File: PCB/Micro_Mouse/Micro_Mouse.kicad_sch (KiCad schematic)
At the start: 12 parts, among them J1 Motor Battery Pack, J3 MOT_1/ENC_1, J4 MOT2/ENC_2, J5 TOF, J6 IR_1, J7 IR_2, J8 IMU, Q1 PMOS, U1 TB6612FNG

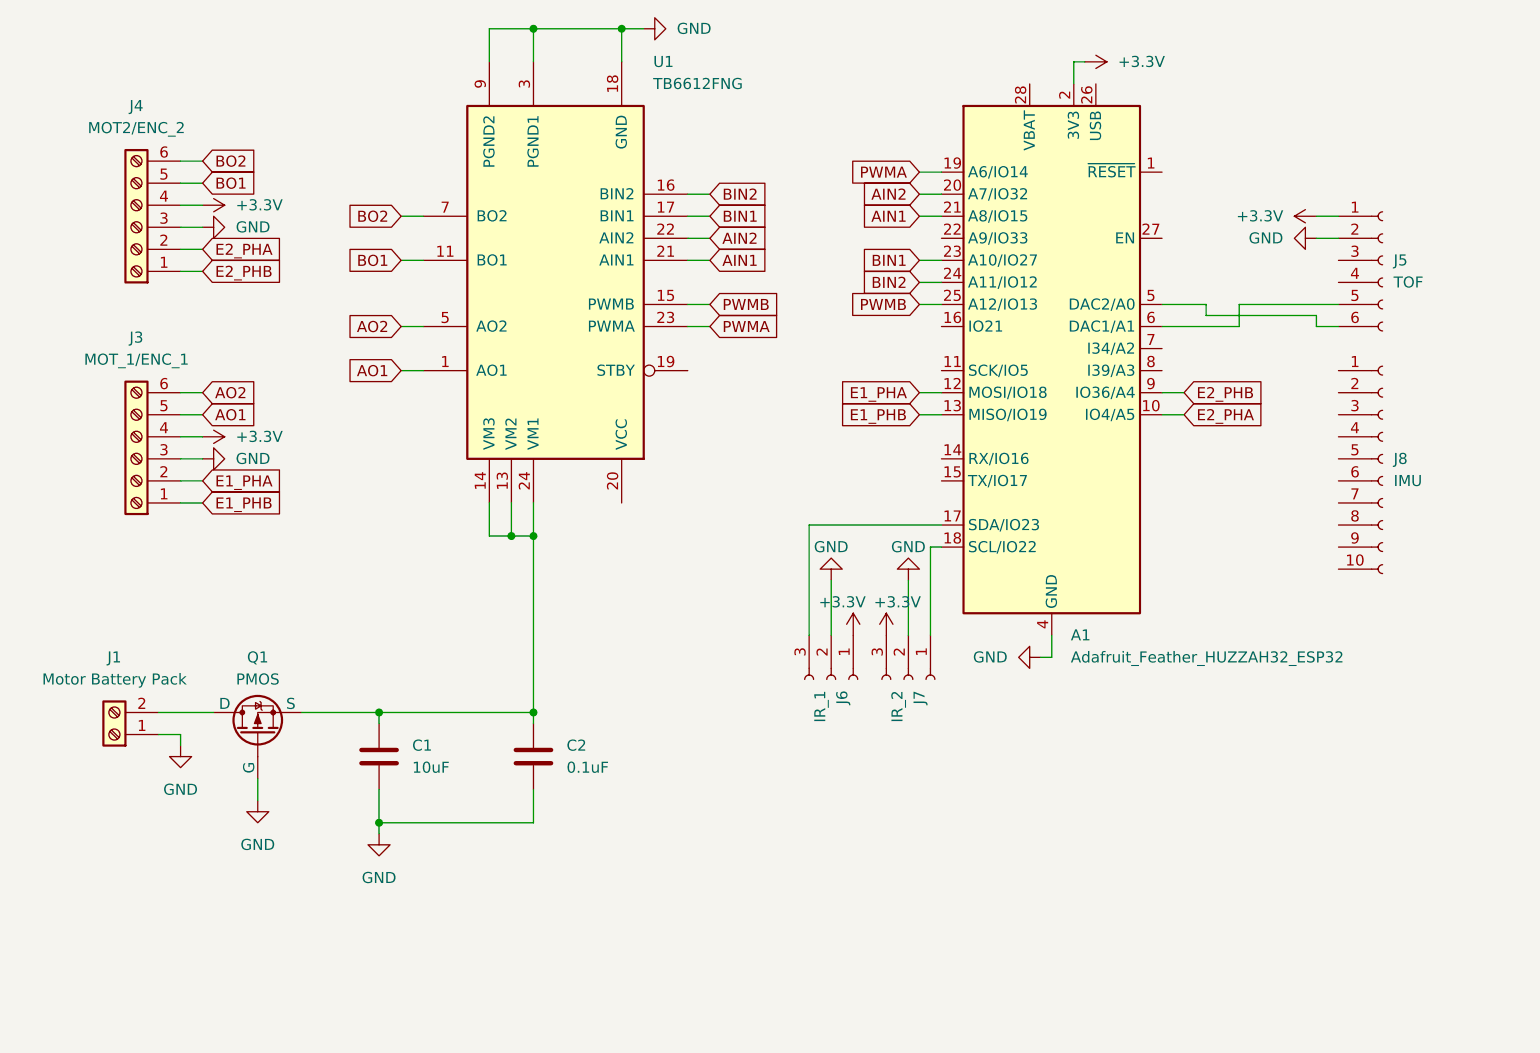
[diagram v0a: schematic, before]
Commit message: Add files via upload
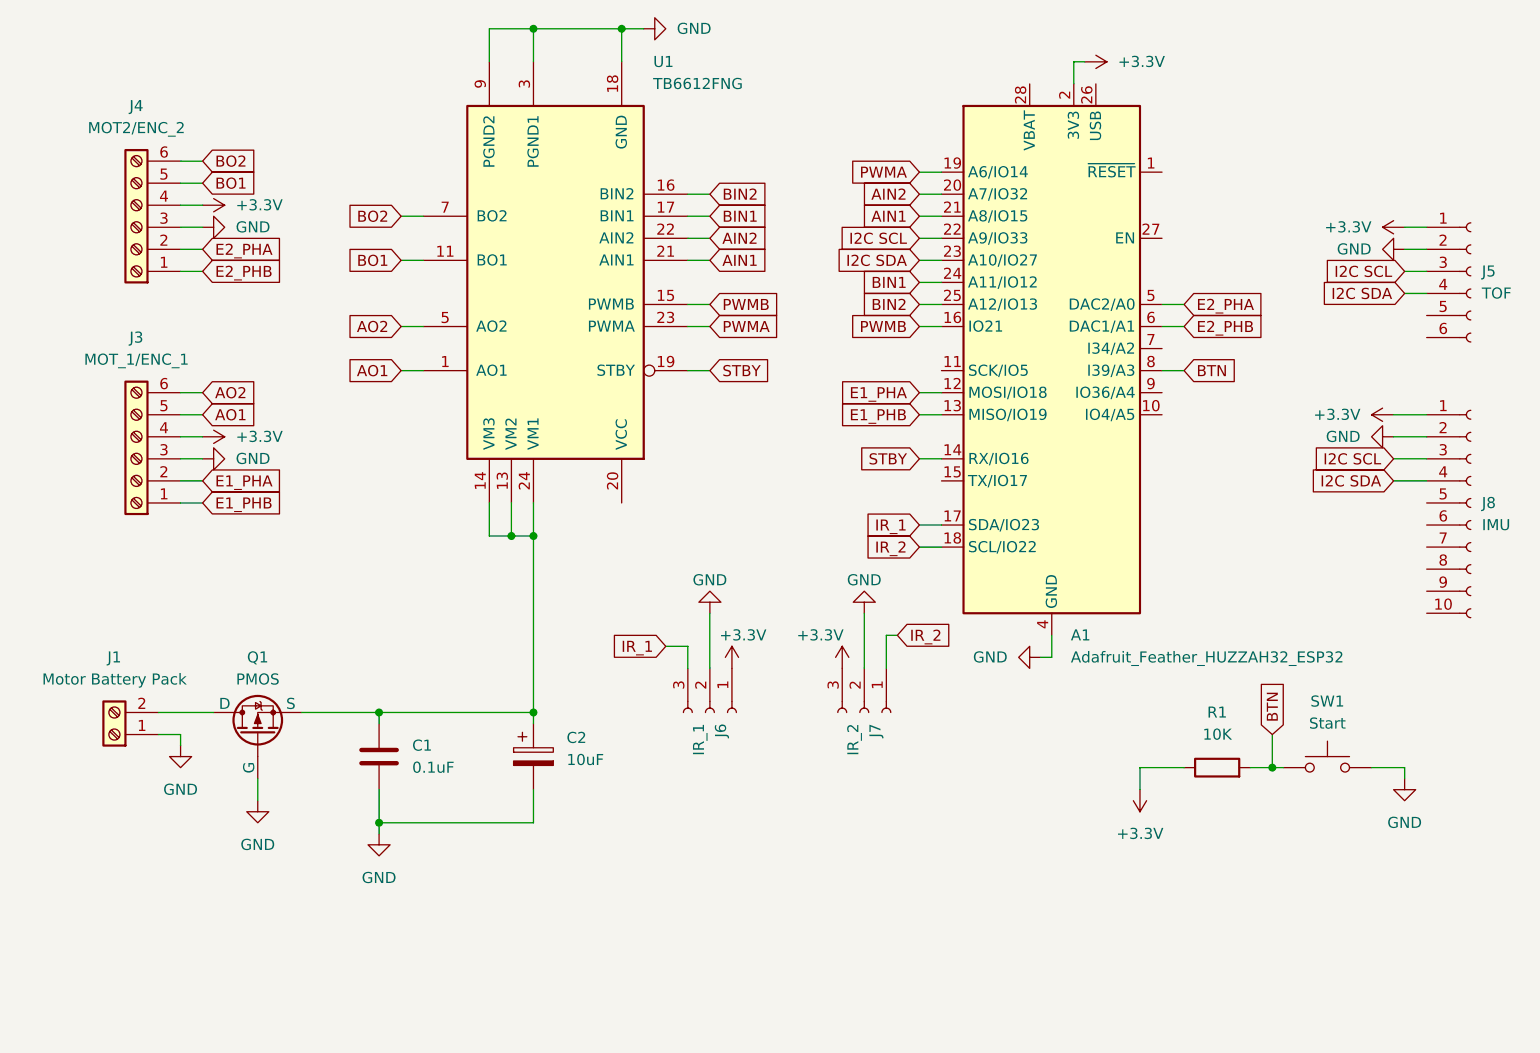
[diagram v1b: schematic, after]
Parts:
- removed C2: 0.1uF, symbol Device:C
- added C2: 10uF, Capacitor_SMD:CP_Elec_3x5.3, symbol Device:C_Polarized
- added R1: 10K, Resistor_SMD:R_0805_2012Metric, symbol Device:R
- added SW1: Start, Button_Switch_SMD:SW_Push_1P1T_NO_CK_KSC6xxJ, symbol Switch:SW_Push
- C1: value 10uF -> 0.1uF; footprint (none) -> Capacitor_SMD:CP_Elec_3x5.3
- J1: footprint TerminalBlock_Phoenix:TerminalBlock_Phoenix_MPT-0,5-2-2.54_1x02_P2.54mm_Horizontal -> Connector_JST:JST_EH_B2B-EH-A_1x02_P2.50mm_Vertical
- Q1: footprint (none) -> Package_TO_SOT_SMD:TO-252-2
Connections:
- net +3.3V: now also J8.1 (Pin_1), R1.1
- net BIN1: now also A1.24 (A11/IO12); no longer A1.23 (A10/IO27)
- net BIN2: now also A1.25 (A12/IO13); no longer A1.24 (A11/IO12)
- net E2_PHA: now also A1.5 (DAC2/A0); no longer A1.10 (IO4/A5)
- net E2_PHB: now also A1.6 (DAC1/A1); no longer A1.9 (IO36/A4)
- net GND: now also J8.2 (Pin_2), C2.2, SW1.2
- net PWMB: now also A1.16 (IO21); no longer A1.25 (A12/IO13)
- net STBY: now reaches A1.14 (RX/IO16)
- net STBY: now also U1.19 (STBY)
- net IR_1: now reaches A1.17 (SDA/IO23), J6.3 (Pin_3)
- net IR_2: now reaches A1.18 (SCL/IO22), J7.1 (Pin_1)
- net I2C SCL: now reaches A1.22 (A9/IO33)
- net I2C SCL: now also J5.3 (Pin_3), J8.3 (Pin_3)
- net at J5.6 (Pin_6): no longer A1.5 (DAC2/A0)
- net at J5.5 (Pin_5): no longer A1.6 (DAC1/A1)
- net BTN: now reaches A1.8 (I39/A3)
- net BTN: now also R1.2, SW1.1
- net at C1.1, Q1.3 (S), U1.13 (VM2)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: now also C2.1
- net I2C SDA: now reaches J8.4 (Pin_4)
- net I2C SDA: now also A1.23 (A10/IO27), J5.4 (Pin_4)
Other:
- title: (none) -> Micro Mouse: Santana, West
- moved on the sheet: J5, J6, J7, J8

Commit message: Add files via upload
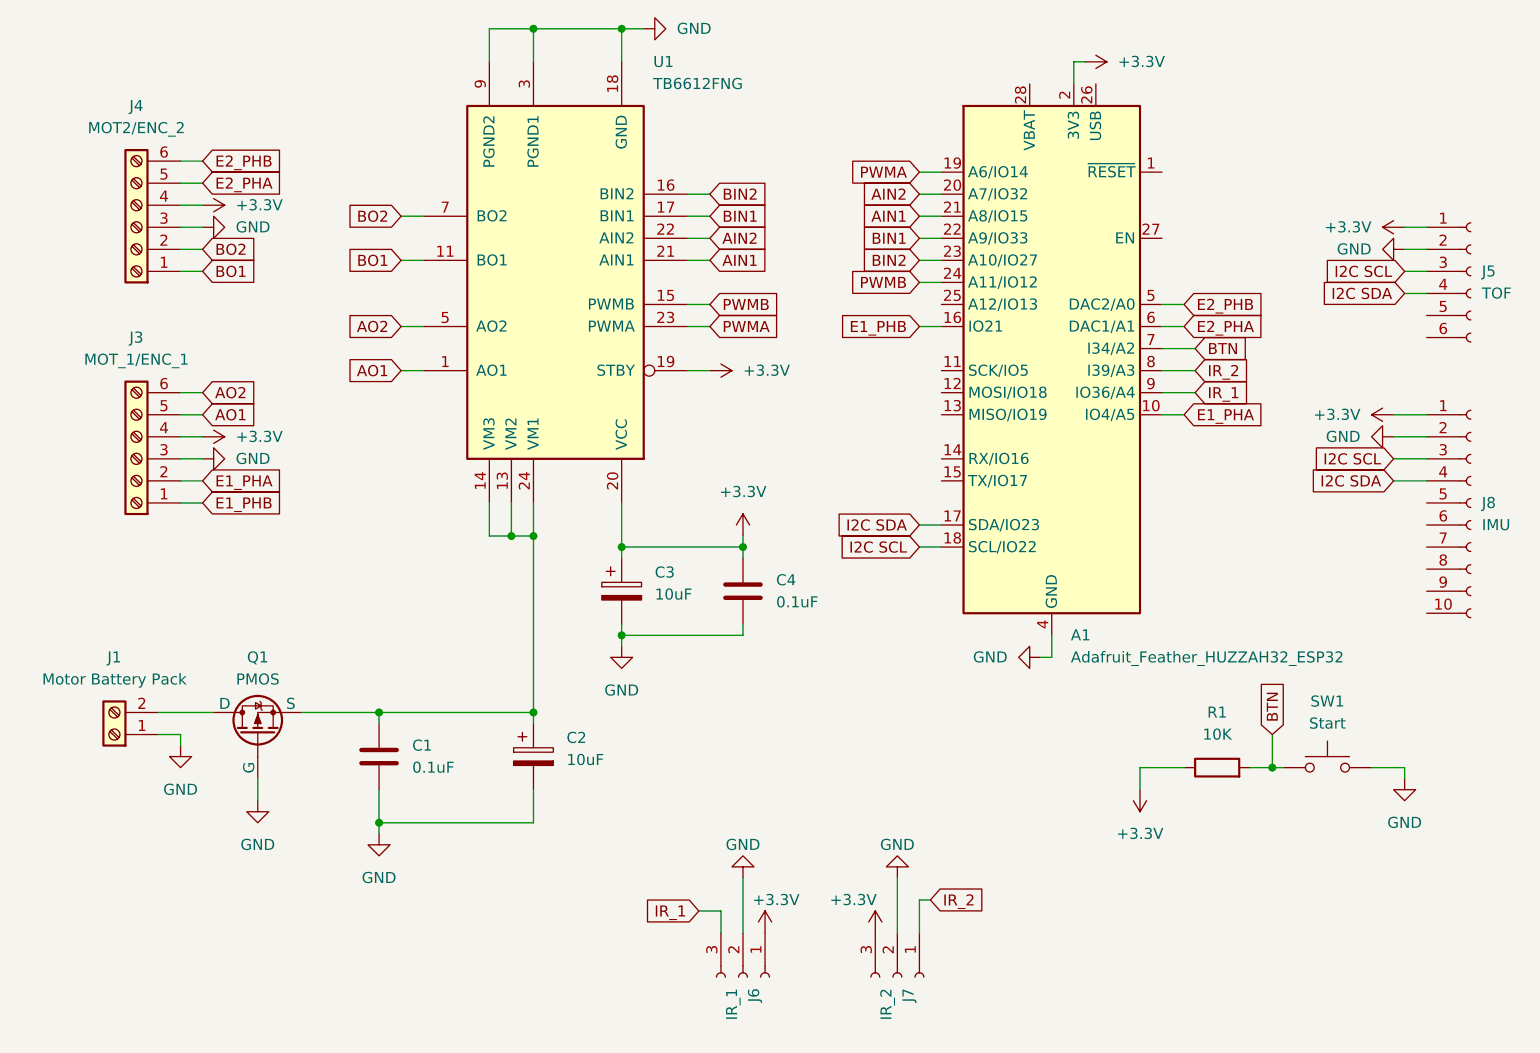
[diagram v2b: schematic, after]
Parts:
- added C3: 10uF, Capacitor_SMD:CP_Elec_3x5.3, symbol Device:C_Polarized
- added C4: 0.1uF, Capacitor_SMD:C_0805_2012Metric_Pad1.18x1.45mm_HandSolder, symbol Device:C
- C1: footprint Capacitor_SMD:CP_Elec_3x5.3 -> Capacitor_SMD:C_0805_2012Metric_Pad1.18x1.45mm_HandSolder
- Q1: footprint Package_TO_SOT_SMD:TO-252-2 -> Package_TO_SOT_SMD:TO-252-3_TabPin2
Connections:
- net +3.3V: now also U1.19 (STBY), U1.20 (VCC), C3.1, C4.1
- net BIN1: now also A1.22 (A9/IO33); no longer A1.24 (A11/IO12)
- net BIN2: now also A1.23 (A10/IO27); no longer A1.25 (A12/IO13)
- net BO1: now also J4.1 (Pin_1); no longer J4.5 (Pin_5)
- net BO2: now also J4.2 (Pin_2); no longer J4.6 (Pin_6)
- net BTN: now also A1.7 (I34/A2); no longer A1.8 (I39/A3)
- net E1_PHA: now also A1.10 (IO4/A5); no longer A1.12 (MOSI/IO18)
- net E1_PHB: now also A1.16 (IO21); no longer A1.13 (MISO/IO19)
- net E2_PHA: now also A1.6 (DAC1/A1), J4.5 (Pin_5); no longer A1.5 (DAC2/A0), J4.2 (Pin_2)
- net E2_PHB: now also A1.5 (DAC2/A0), J4.6 (Pin_6); no longer A1.6 (DAC1/A1), J4.1 (Pin_1)
- net GND: now also C3.2, C4.2
- net I2C SCL: now also A1.18 (SCL/IO22); no longer A1.22 (A9/IO33)
- net I2C SDA: now also A1.17 (SDA/IO23); no longer A1.23 (A10/IO27)
- net IR_1: now also A1.9 (IO36/A4); no longer A1.17 (SDA/IO23)
- net IR_2: now also A1.8 (I39/A3); no longer A1.18 (SCL/IO22)
- net PWMB: now also A1.24 (A11/IO12); no longer A1.16 (IO21)
- net STBY: no longer names the net of A1.14 (RX/IO16)
- net STBY: no longer U1.19 (STBY)
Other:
- moved on the sheet: J6, J7

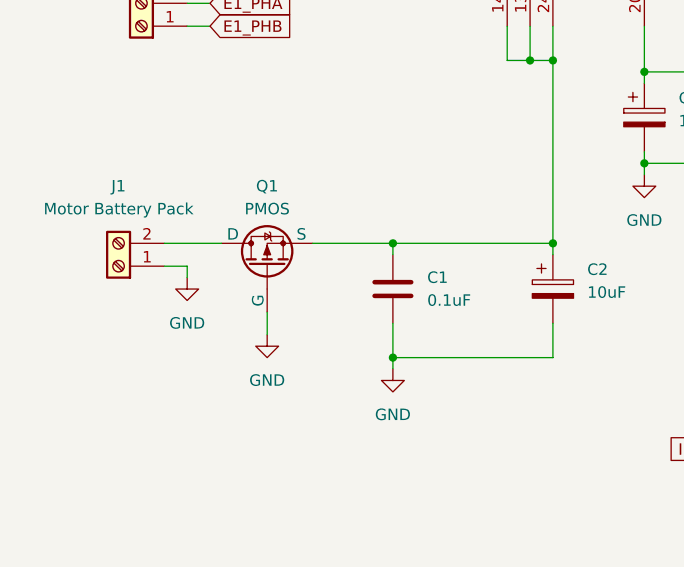
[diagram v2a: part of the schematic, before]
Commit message: Add files via upload
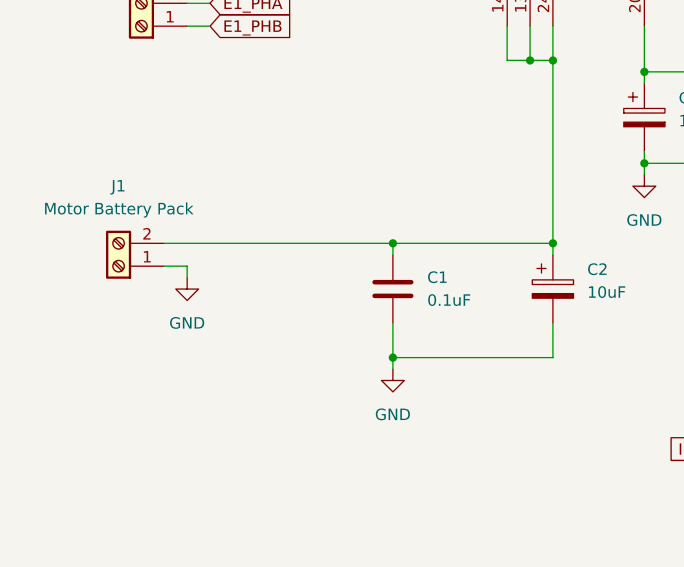
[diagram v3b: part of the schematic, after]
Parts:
- removed Q1: PMOS, Package_TO_SOT_SMD:TO-252-3_TabPin2, symbol Simulation_SPICE:PMOS
- J4: footprint TerminalBlock_Phoenix:TerminalBlock_Phoenix_MPT-0,5-6-2.54_1x06_P2.54mm_Horizontal -> Connector_JST:JST_ZE_B06B-ZESK-1D_1x06_P1.50mm_Vertical
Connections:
- net at C1.1, C2.1, U1.13 (VM2)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: now also J1.2 (Pin_2)
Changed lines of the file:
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@@
     (stroke (width 0) (type default))
   )
-  (wire (pts (xy 59.69 137.16) (xy 68.58 137.16))
+  (wire (pts (xy 43.18 137.16) (xy 68.58 137.16))
     (stroke (width 0) (type default))
   )
@@
     (stroke (width 0) (type default))
   )
-  (wire (pts (xy 43.18 137.16) (xy 49.53 137.16))
-    (stroke (width 0) (type default))
-  )
   (wire (pts (xy 110.49 127) (xy 110.49 128.27))
     (stroke (width 0) (type default))
@@
   )
   (wire (pts (xy 171.45 143.51) (xy 172.72 143.51))
-    (stroke (width 0) (type default))
-  )
-  (wire (pts (xy 54.61 144.78) (xy 54.61 147.32))
     (stroke (width 0) (type default))
   )
@@
     )
   )
-  (symbol (lib_id "power:GND") (at 54.61 147.32 0) (unit 1)
-    (in_bom yes) (on_board yes) (dnp no) (fields_autoplaced)
-    (property "Reference" "#PWR010" (at 54.61 153.67 0)
-      (effects (font (size 1.27 1.27)) hide)
-    )
-    (property "Value" "GND" (at 54.61 152.4 0)
-      (effects (font (size 1.27 1.27)))
-    )
-    (property "Footprint" "" (at 54.61 147.32 0)
-      (effects (font (size 1.27 1.27)) hide)
-    )
-    (property "Datasheet" "" (at 54.61 147.32 0)
-      (effects (font (size 1.27 1.27)) hide)
-    )
-    (pin "1")
-    (instances
-      (project "Micro_Mouse"
-        (path "/2f5422af-6937-496c-8d34-480d197513da"
-          (reference "#PWR010") (unit 1)
-        )
-      )
-    )
-  )
   (symbol (lib_id "Driver_Motor:TB6612FNG") (at 88.9 87.63 180) (unit 1)
     (in_bom yes) (on_board yes) (dnp no) (fields_autoplaced)
@@
     )
   )
-  (symbol (lib_id "Simulation_SPICE:PMOS") (at 54.61 139.7 90) (unit 1)
-    (in_bom yes) (on_board yes) (dnp no) (fields_autoplaced)
-    (property "Reference" "Q1" (at 54.61 130.81 90)
-      (effects (font (size 1.27 1.27)))
-    )
-    (property "Value" "PMOS" (at 54.61 133.35 90)
-      (effects (font (size 1.27 1.27)))
-    )
-    (property "Footprint" "Package_TO_SOT_SMD:TO-252-3_TabPin2" (at 52.07 134.62 0)
-      (effects (font (size 1.27 1.27)) hide)
-    )
-    (property "Datasheet" "https://ngspice.sourceforge.io/docs/ngspice-manual.pdf" (at 67.31 139.7 0)
-      (effects (font (size 1.27 1.27)) hide)
-    )
-    (property "Sim.Device" "PMOS" (at 71.755 139.7 0)
-      (effects (font (size 1.27 1.27)) hide)
-    )
-    (property "Sim.Type" "VDMOS" (at 73.66 139.7 0)
-      (effects (font (size 1.27 1.27)) hide)
-    )
-    (property "Sim.Pins" "1=D 2=G 3=S" (at 69.85 139.7 0)
-      (effects (font (size 1.27 1.27)) hide)
-    )
-    (pin "1")
-    (pin "2")
-    (pin "3")
-    (instances
-      (project "Micro_Mouse"
-        (path "/2f5422af-6937-496c-8d34-480d197513da"
-          (reference "Q1") (unit 1)
-        )
-      )
-    )
-  )
   (symbol (lib_id "Switch:SW_Push") (at 177.8 143.51 0) (unit 1)
     (in_bom yes) (on_board yes) (dnp no) (fields_autoplaced)
@@
       (effects (font (size 1.27 1.27)))
     )
-    (property "Footprint" "TerminalBlock_Phoenix:TerminalBlock_Phoenix_MPT-0,5-6-2.54_1x06_P2.54mm_Horizontal" (at 40.64 81.28 0)
-      (effects (font (size 1.27 1.27)) hide)
-    )
+    (property "Footprint" "Connector_JST:JST_ZE_B06B-ZESK-1D_1x06_P1.50mm_Vertical" (at 40.64 81.28 0)
+      (effects (font (size 1.27 1.27)) hide)
+    )
